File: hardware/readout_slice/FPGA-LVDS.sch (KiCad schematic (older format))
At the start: 8 parts

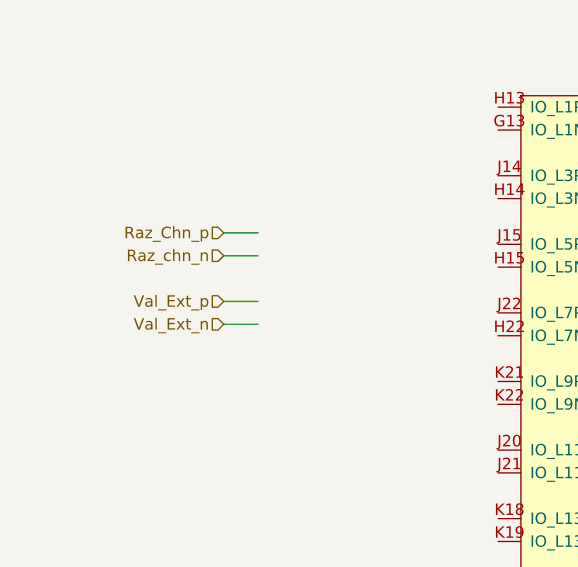
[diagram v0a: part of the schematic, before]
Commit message: auto push run at Tue Apr 20 18:13:16 EDT 2021
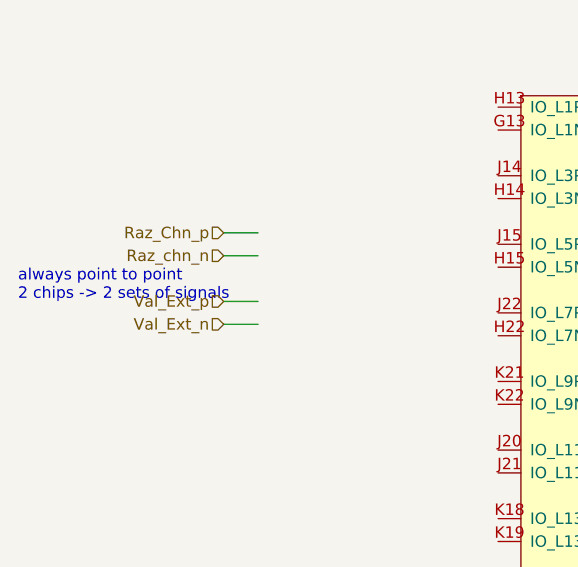
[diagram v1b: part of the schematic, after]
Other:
- note added: "always point to point\n2 chips -> 2 sets of signals"
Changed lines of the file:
@@
 Wire Wire Line
 	1650 3650 1800 3650
+Text Notes 750  3550 0    50   ~ 0
+always point to point\n2 chips -> 2 sets of signals
 $EndSCHEMATC

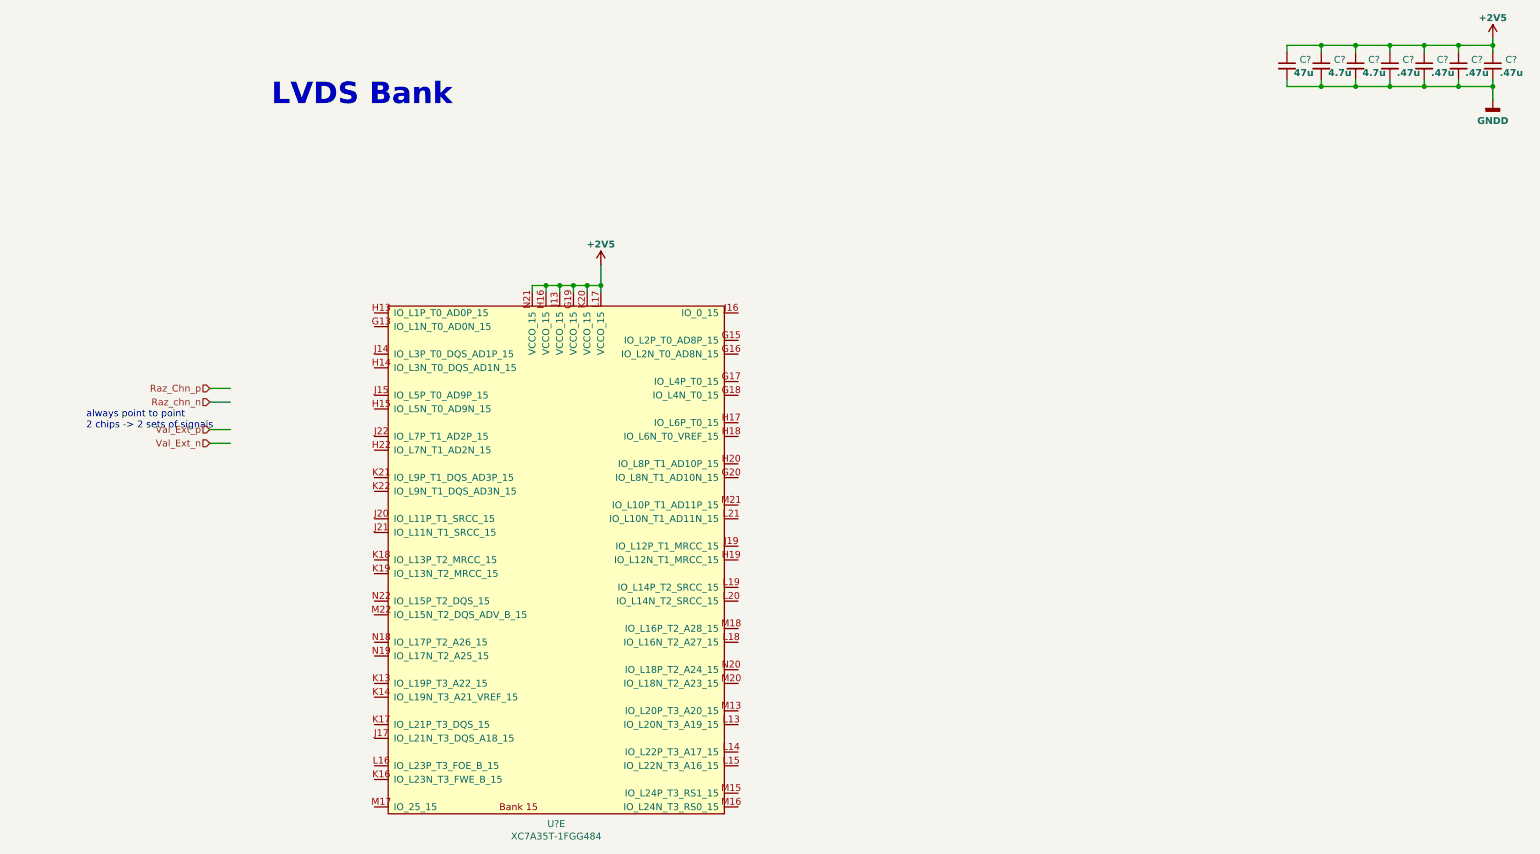
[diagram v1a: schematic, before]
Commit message: auto push run at Wed Apr 21 10:59:57 EDT 2021
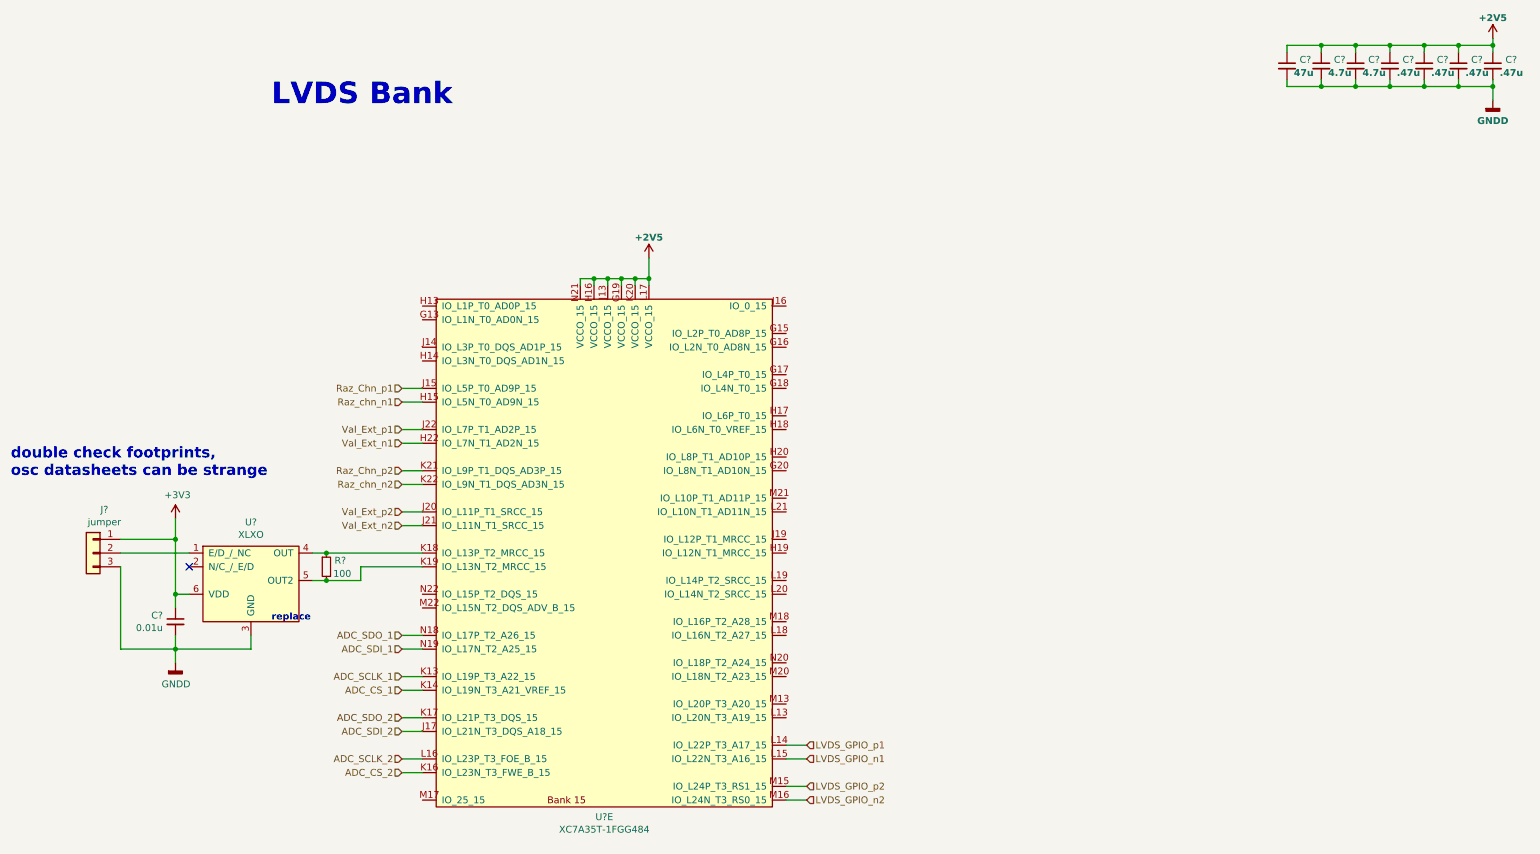
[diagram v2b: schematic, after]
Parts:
- added C?: 0.01u, symbol Device:C_Small
- added J?: jumper, symbol Connector_Generic:Conn_01x03
- added R?: 100, symbol Device:R_Small
- added U?: XLXO, symbol readout:XLXO
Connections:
- net labels added: +3V3, ADC_CS_1, ADC_CS_2, ADC_SCLK_1, ADC_SCLK_2, ADC_SDI_1, ADC_SDI_2, ADC_SDO_1, ADC_SDO_2, LVDS_GPIO_n1, LVDS_GPIO_n2, LVDS_GPIO_p1, LVDS_GPIO_p2, Raz_Chn_p1, Raz_Chn_p2, Raz_chn_n1, Raz_chn_n2, Val_Ext_n1, Val_Ext_n2, Val_Ext_p1, Val_Ext_p2
- net labels removed: Raz_Chn_p, Raz_chn_n, Val_Ext_n, Val_Ext_p
- wire segments 44 -> 78
- no-connect marks 0 -> 1
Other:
- note added: "double check footprints,\nosc datasheets can be strange"
- note added: "replace\n"
- note removed: "always point to point\n2 chips -> 2 sets of signals"
- moved on the sheet: U?E
